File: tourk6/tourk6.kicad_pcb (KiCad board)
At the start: 2 copper layers, 30.5 x 20.3 mm, 5 parts, among them J1 Conn_01x03

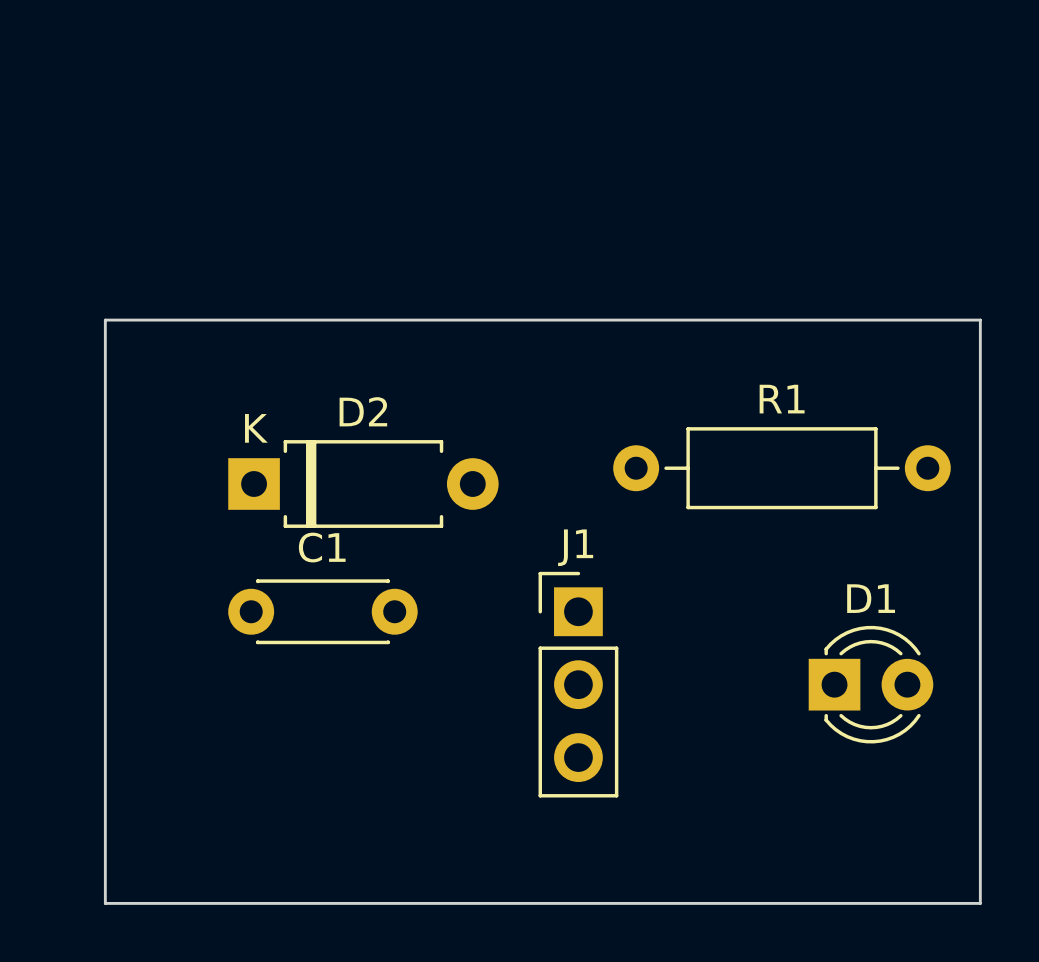
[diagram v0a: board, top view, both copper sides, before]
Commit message: Avances en el PCB.
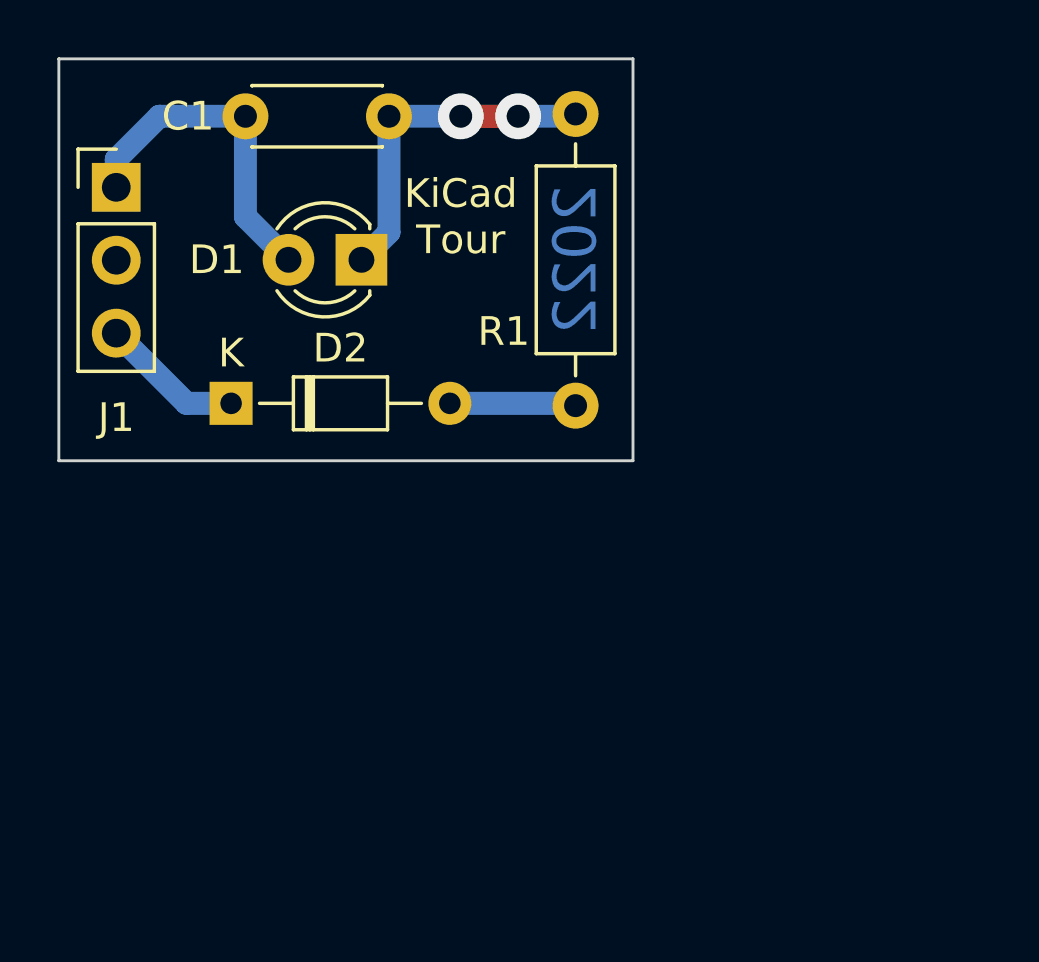
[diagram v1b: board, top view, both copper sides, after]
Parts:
- D2: footprint Diode_THT:D_A-405_P7.62mm_Horizontal -> Diode_THT:D_DO-34_SOD68_P7.62mm_Horizontal
- moved D1 22.2 mm to (143.5, 99.5), turned to 180 degrees
- moved J1 21.9 mm to (135.0, 97.0)
- moved C1 17.3 mm to (139.5, 94.5)
- moved R1 12.5 mm to (151.0, 94.4), turned to -90 degrees
- moved D2 2.92 mm to (139.0, 104.5)
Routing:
- net Net-(C1-Pad2): track 0.00 -> 11.9 mm, vias 0 -> 2
- net Net-(C1-Pad1): track 0.00 -> 11.7 mm
- net Net-(D2-Pad1): track 0.00 -> 5.01 mm
- net Net-(D2-Pad2): track 0.00 -> 4.41 mm
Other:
- board size 30.5 x 20.3 mm -> 20 x 14 mm
- board text added: "2022"
- board text added: "KiCad Tour"
